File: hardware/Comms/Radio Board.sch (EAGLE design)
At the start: 1 part

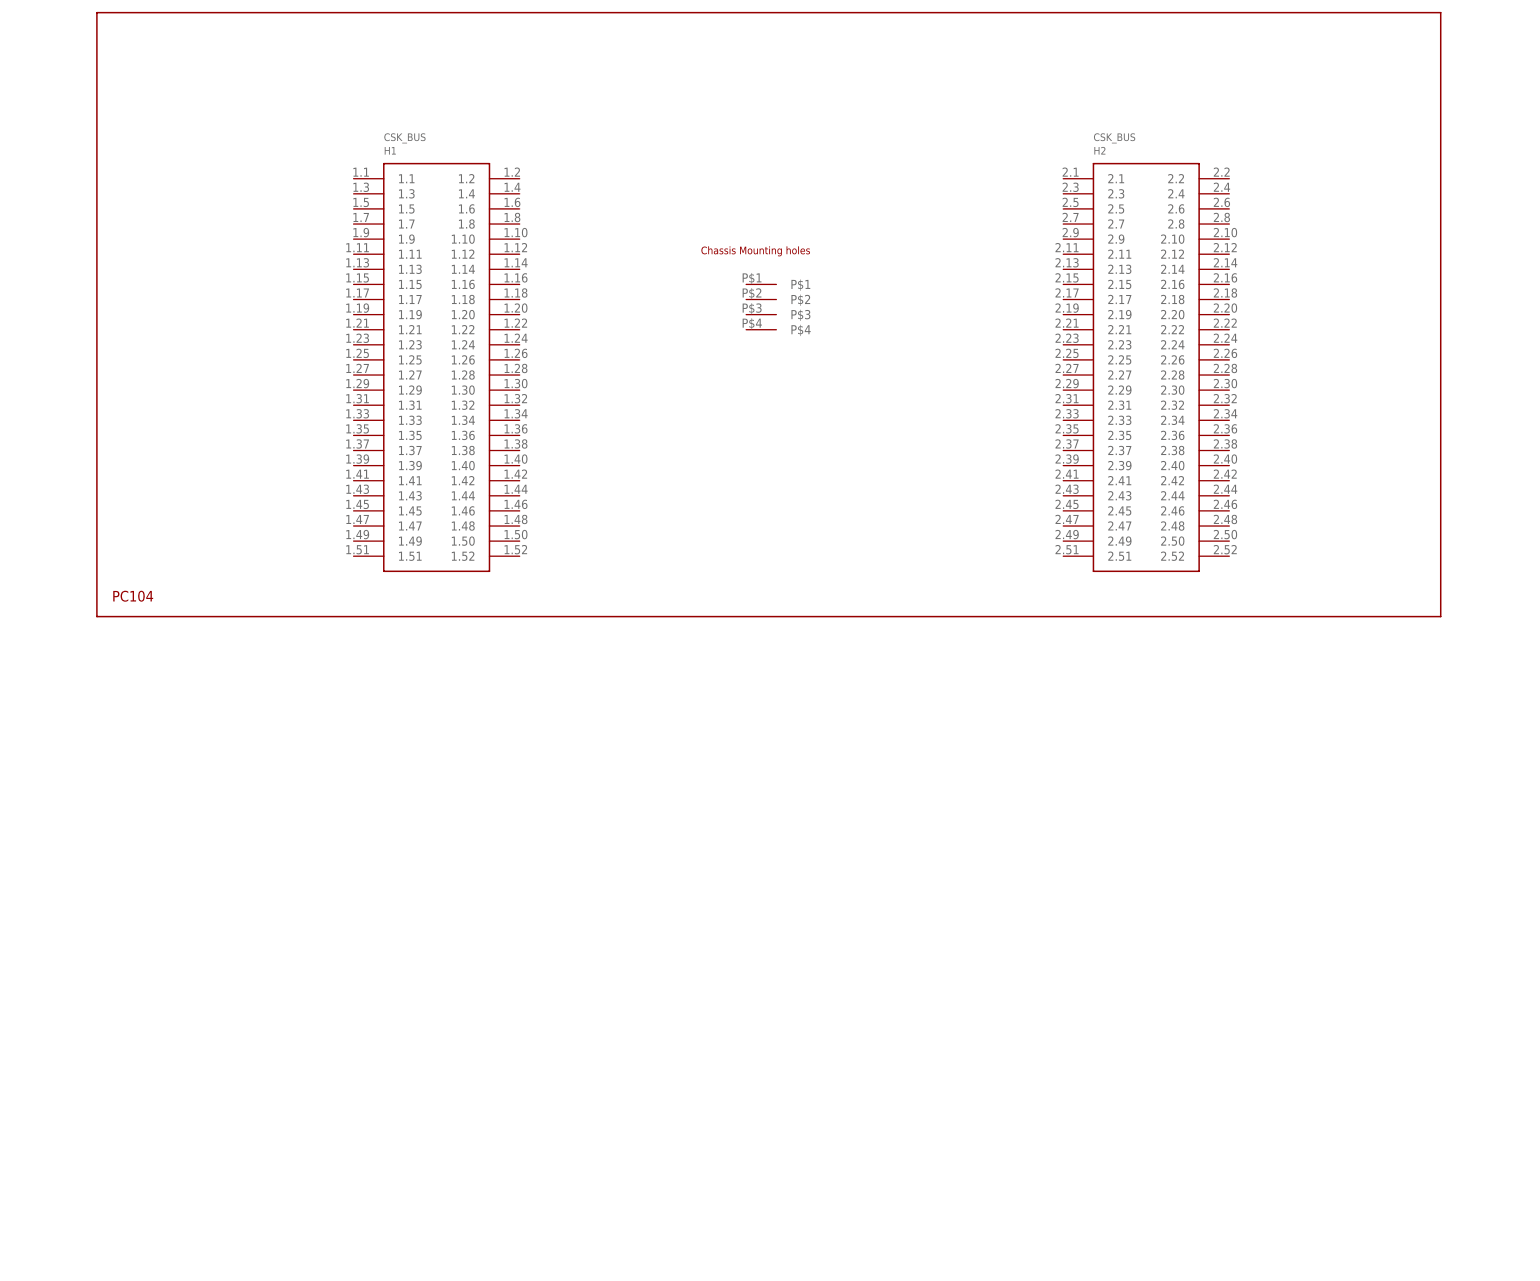
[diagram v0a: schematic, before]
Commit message: Completed radio boards
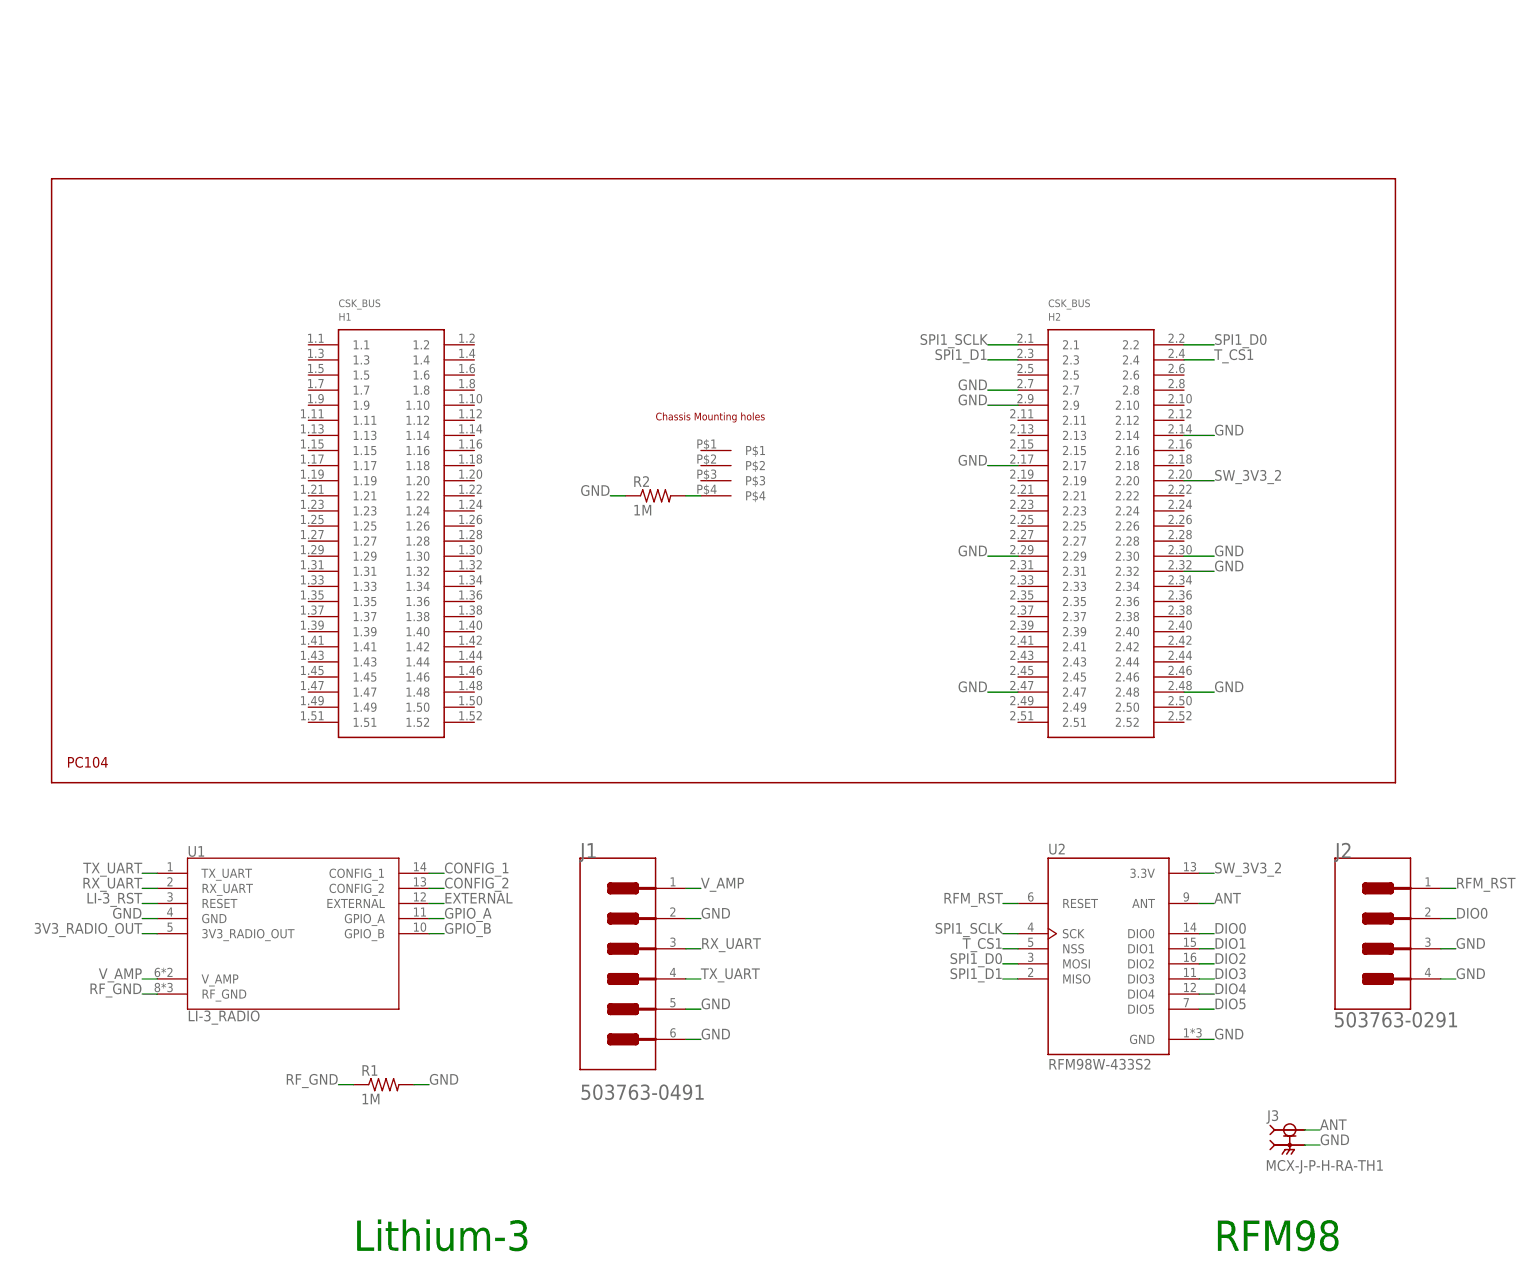
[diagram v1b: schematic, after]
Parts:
- added J1: MOLEX_503763-0491MOLEX_503763-0491_0_0, Molex - 503763-0491:MOLEX_503763-0491MOLEX_503763-0491_0_0
- added J2: MOLEX_503763-0291MOLEX_503763-0291_0_0, Molex - 503763-0291:MOLEX_503763-0291MOLEX_503763-0291_0_0
- added J3: MCX-J-P-H-RA-TH1, MCX-J-P-H-RA-TH1:MCX-J-P-H-RA-TH1
- added R1, R2: 1M, HSFL_Main_Library:RESISTOR0805-RES
- added U1: LI-3_RADIO, Lithium-3 Radio:LI-3_RADIO
- added U2: RFM98W-433S2, RFM98:RFM98W-433S2
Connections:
- new net 3V3_RADIO_OUT: U1.3V3_RADIO_OUT
- new net ANT: J3.1, U2.ANT
- new net CONFIG_1: U1.CONFIG_1
- new net CONFIG_2: U1.CONFIG_2
- new net DIO0: J2.2, U2.DIO0
- new net DIO1: U2.DIO1
- new net DIO2: U2.DIO2
- new net DIO3: U2.DIO3
- new net DIO4: U2.DIO4
- new net DIO5: U2.DIO5
- new net EXTERNAL: U1.EXTERNAL
- new net GND: H1.2.14, H1.2.17, H1.2.29, H1.2.30, H1.2.32, H1.2.47, H1.2.48, H1.2.7, H1.2.9, J1.2, J1.MNT_1, J1.MNT_2, J2.MNT_1, J2.MNT_2, J3.2, R1.2, R2.1, U1.GND, U2.GND
- new net GPIO_A: U1.GPIO_A
- new net GPIO_B: U1.GPIO_B
- new net LI-3_RST: U1.RESET
- new net N$1: H1.P$4, R2.2
- new net RFM_RST: J2.1, U2.RESET
- new net RF_GND: R1.1, U1.RF_GND
- new net RX_UART: J1.3, U1.RX_UART
- new net SPI1_D0: H1.2.2, U2.MOSI
- new net SPI1_D1: H1.2.3, U2.MISO
- new net SPI1_SCLK: H1.2.1, U2.SCK
- new net SW_3V3_2: H1.2.20, U2.3.3V
- new net TX_UART: J1.4, U1.TX_UART
- new net T_CS1: H1.2.4, U2.NSS
- new net V_AMP: J1.1, U1.V_AMP
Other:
- note added: "Lithium-3"
- note added: "RFM98"
